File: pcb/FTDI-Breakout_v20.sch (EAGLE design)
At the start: 35 parts, among them IC1 FT231XQ, IC2 LDO-TS5204-3V3, X1 PASSER-07, X2 PASSER-07

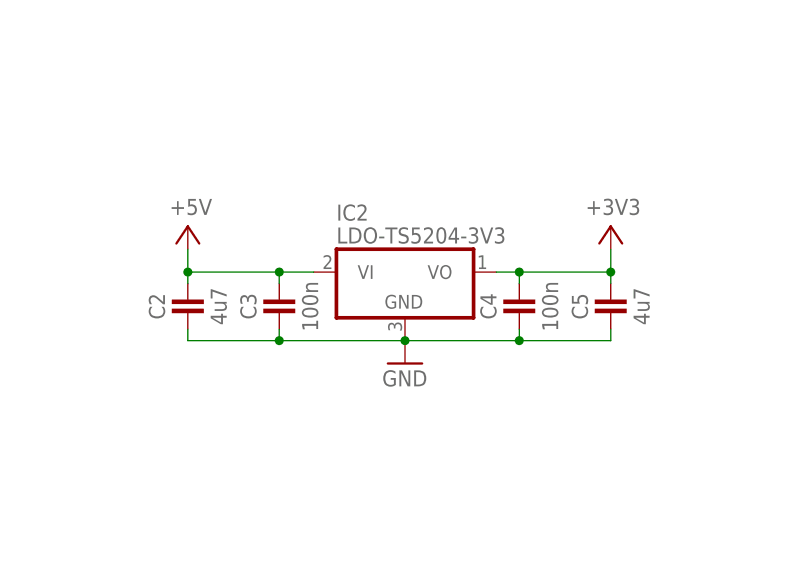
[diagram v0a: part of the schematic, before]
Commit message: updated schematics and layout
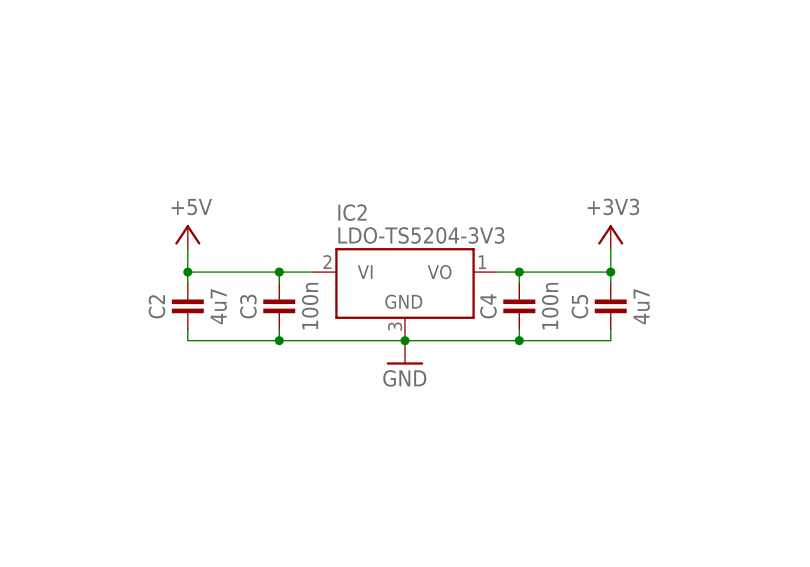
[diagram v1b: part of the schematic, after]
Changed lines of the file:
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@@
 <layer number="154" name="FabDoc2" color="2" fill="1" visible="no" active="no"/>
 <layer number="155" name="FabDoc3" color="7" fill="15" visible="no" active="no"/>
+<layer number="200" name="200bmp" color="1" fill="10" visible="no" active="no"/>
 <layer number="217" name="217bmp" color="18" fill="1" visible="no" active="no"/>
 <layer number="218" name="218bmp" color="19" fill="1" visible="no" active="no"/>
